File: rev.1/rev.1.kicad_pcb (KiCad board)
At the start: 2 copper layers, 100 x 100 mm, 129 parts, among them Q1 BC857, Q2 BC817, SW1 RESET, SW2 POWER, X1 POWER, X2 Манипулятор_1, X3 AUDIO_1, X4 AUDIO_2, X5 Манипулятор_2, X6 VIDEO

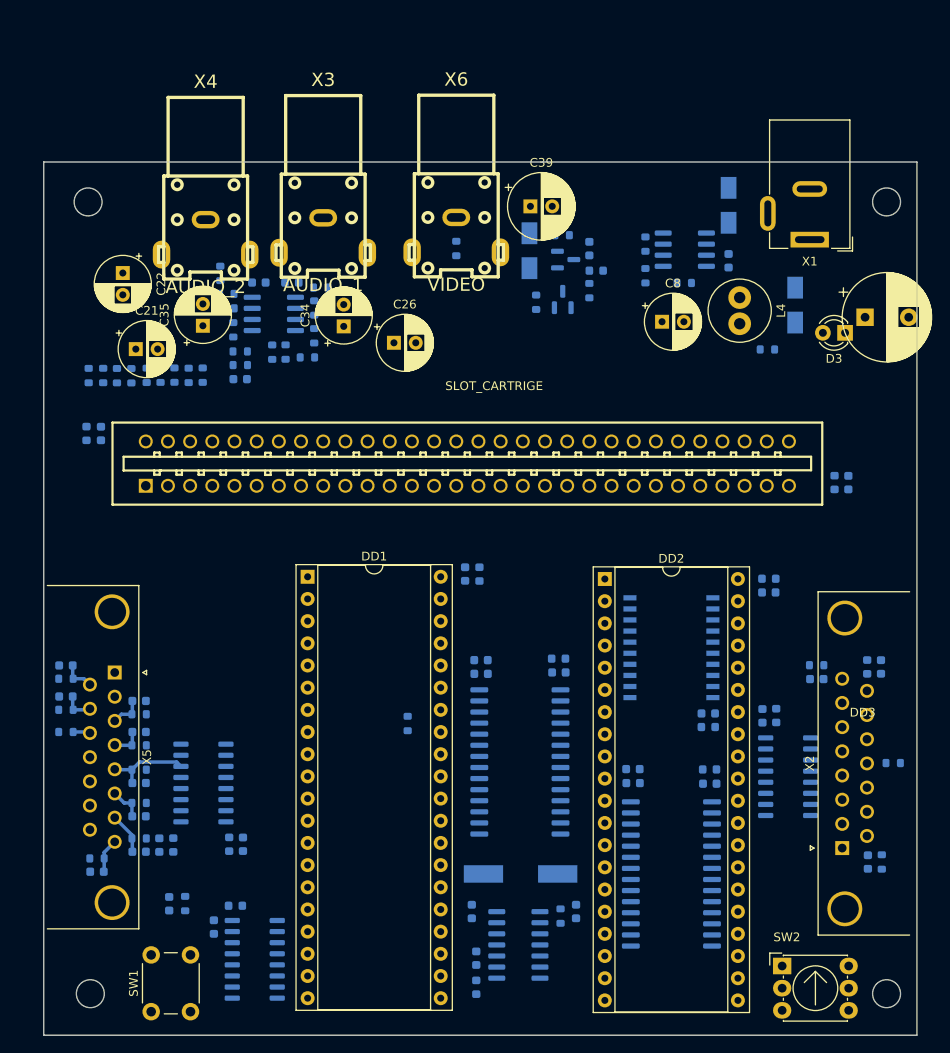
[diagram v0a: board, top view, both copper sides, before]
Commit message: Сделал разводку печатной платы
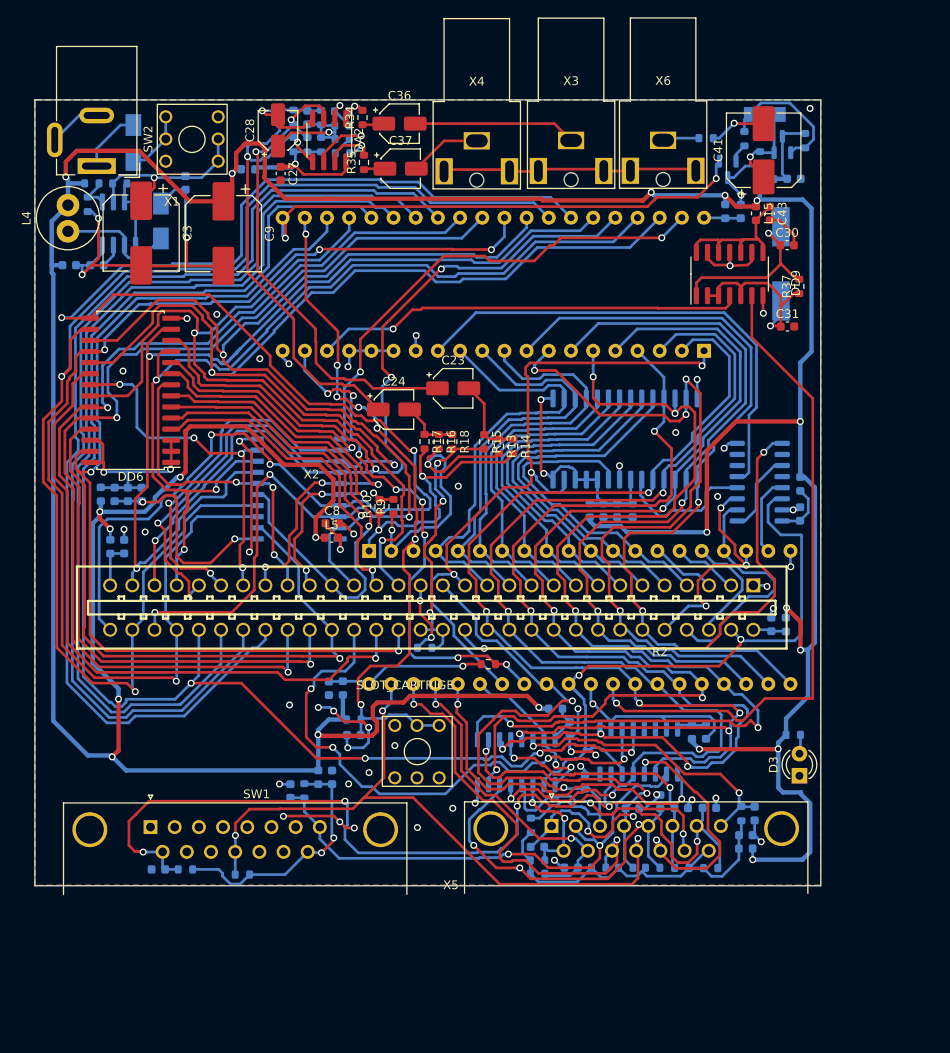
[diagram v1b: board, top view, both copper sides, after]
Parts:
- added C10: 0.1uF, Capacitor_SMD:C_0603_1608Metric, B.Cu at (24.2, 59.6)
- added C2: 0.1uF, Capacitor_SMD:C_0603_1608Metric, B.Cu at (37.6, 50.1)
- C23: renamed from C21; footprint Capacitor_THT:CP_Radial_D6.3mm_P2.50mm -> Capacitor_SMD:CP_Elec_4x5.4
- C24: renamed from C22; footprint Capacitor_THT:CP_Radial_D6.3mm_P2.50mm -> Capacitor_SMD:CP_Elec_4x5.4
- C27: renamed from C25; moved to F.Cu
- C28: renamed from C26; footprint Capacitor_THT:CP_Radial_D6.3mm_P2.50mm -> Capacitor_SMD:CP_Elec_4x5.4
- C3: renamed from C2; footprint Capacitor_THT:CP_Radial_D10.0mm_P5.00mm -> Capacitor_SMD:CP_Elec_8x10.5
- C30: renamed from C28; moved to F.Cu
- C31: renamed from C29; moved to F.Cu
- C36: renamed from C34; footprint Capacitor_THT:CP_Radial_D6.3mm_P2.50mm -> Capacitor_SMD:CP_Elec_4x5.4
- C37: renamed from C35; footprint Capacitor_THT:CP_Radial_D6.3mm_P2.50mm -> Capacitor_SMD:CP_Elec_4x5.4
- C41: renamed from C39; footprint Capacitor_THT:CP_Radial_D7.5mm_P2.50mm -> Capacitor_SMD:CP_Elec_8x6.5
- C43: renamed from C41; moved to F.Cu
- C8: renamed from C7; moved to F.Cu
- C9: renamed from C8; footprint Capacitor_THT:CP_Radial_D6.3mm_P2.50mm -> Capacitor_SMD:CP_Elec_8x10.5
- D4: value SS14 -> BAS85; footprint Diode_SMD:D_SMA -> Diode_SMD:D_MiniMELF
- DA2, DD6, DD9, L15, L5, R10, R13, R14, R15, R16, R17, R18, R2, R34, R35, R37, R9: moved to F.Cu
- DD1, DD2: moved to B.Cu
- SW1: footprint Button_Switch_THT:SW_PUSH_6mm_H7.3mm -> Button_Switch_THT:KLS7_P8X8
- SW2: footprint Button_Switch_THT:Nidec_Copal_SH-7010C -> Button_Switch_THT:KLS7_P8X8
- X3, X4, X6: footprint Connector_Audio:rca_red -> Connector_Audio:RCA-105
- moved SW2 116.1 mm to (35.3, 47.7), turned to 90 degrees
- moved L15 94.2 mm to (102.9, 53.6), turned to -90 degrees
- moved C43 91.7 mm to (104.5, 53.6), turned to -90 degrees
- moved C30 84.4 mm to (106.5, 57.3), turned to 0 degrees
- moved C3 83.5 mm to (32.5, 55.9), turned to -90 degrees
- moved C19 83.3 mm to (30.5, 91.8)
- moved L10 83.3 mm to (29.0, 91.8)
- moved DD6 83.1 mm to (31.3, 73.9)
- moved L12 83.0 mm to (106.3, 100.7)
- moved C6 82.1 mm to (108.0, 88.1), turned to 90 degrees
- moved X1 82.1 mm to (27.4, 48.2)
- moved C21 81.3 mm to (34.5, 128.8), turned to 180 degrees
- moved L3 80.7 mm to (108.0, 84.6), turned to -90 degrees
- moved DD9 80.5 mm to (99.9, 60.6), turned to 90 degrees
- moved C25 79.8 mm to (104.7, 100.7)
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- renumbered C9 to C11, C10 to C12, C11 to C13, C12 to C14, C13 to C15, C14 to C16, C15 to C17, C16 to C18, C17 to C19, C18 to C20, C19 to C21, C20 to C22, C23 to C25, C24 to C26, C27 to C29, C30 to C32, C31 to C33, C32 to C34, C33 to C35, C36 to C38, C37 to C39, C3 to C4, C38 to C40, C40 to C42, C42 to C44, C4 to C5, C5 to C6, C6 to C7
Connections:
- SW1 pad 1: GNDD -> unconnected-(SW1-Pad1)
- SW1 pad 2: /RESET -> GNDD
- SW2 pad 1: Net-(D1-K) -> unconnected-(SW2-Pad1)
- SW2 pad 2: Net-(DA1-Vin) -> Net-(D1-K)
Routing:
- net +5V: track 0.00 -> 473.5 mm, vias 0 -> 20
- net GNDD: track 0.00 -> 287.9 mm, vias 0 -> 62
- net /PAD4: track 0.00 -> 188.1 mm, vias 0 -> 4
- net /PA13: track 0.00 -> 162.2 mm, vias 0 -> 4
- net /PAD0: track 0.00 -> 157.1 mm, vias 0 -> 4
- net /PAD5: track 0.00 -> 154.8 mm, vias 0 -> 2
- net /PAD6: track 0.00 -> 144.2 mm, vias 0 -> 4
- net /PAD7: track 0.00 -> 135.2 mm, vias 0 -> 4
- net /D0: track 0.00 -> 135.1 mm, vias 0 -> 6
- net /D1: track 0.00 -> 126.1 mm, vias 0 -> 4
- net /PAD2: track 0.00 -> 125.4 mm, vias 0 -> 4
- net /PA10: track 0.00 -> 123.7 mm
- net /D4: track 0.00 -> 120.3 mm, vias 0 -> 5
- net /D3: track 0.00 -> 119.4 mm, vias 0 -> 4
- net /PA8: track 0.00 -> 119.0 mm, vias 0 -> 2
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- added copper zone on B.Cu, net GNDD
- added copper zone on F.Cu, net GNDD
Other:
- board size 100 x 100 mm -> 90 x 90 mm
